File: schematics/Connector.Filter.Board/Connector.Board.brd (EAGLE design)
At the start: 160 x 100 mm, 43 parts

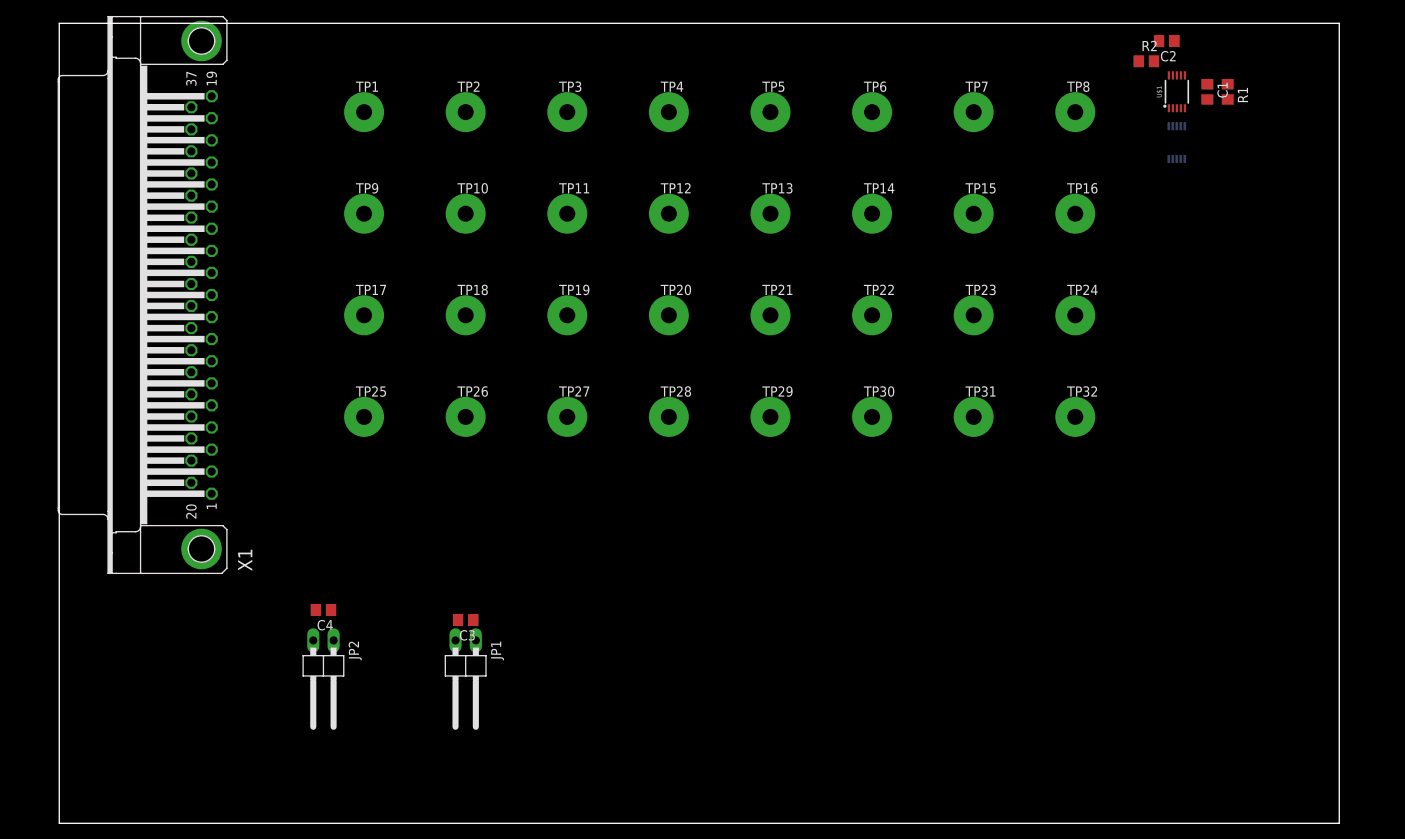
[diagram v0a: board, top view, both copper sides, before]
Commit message: example layout for 4 channels
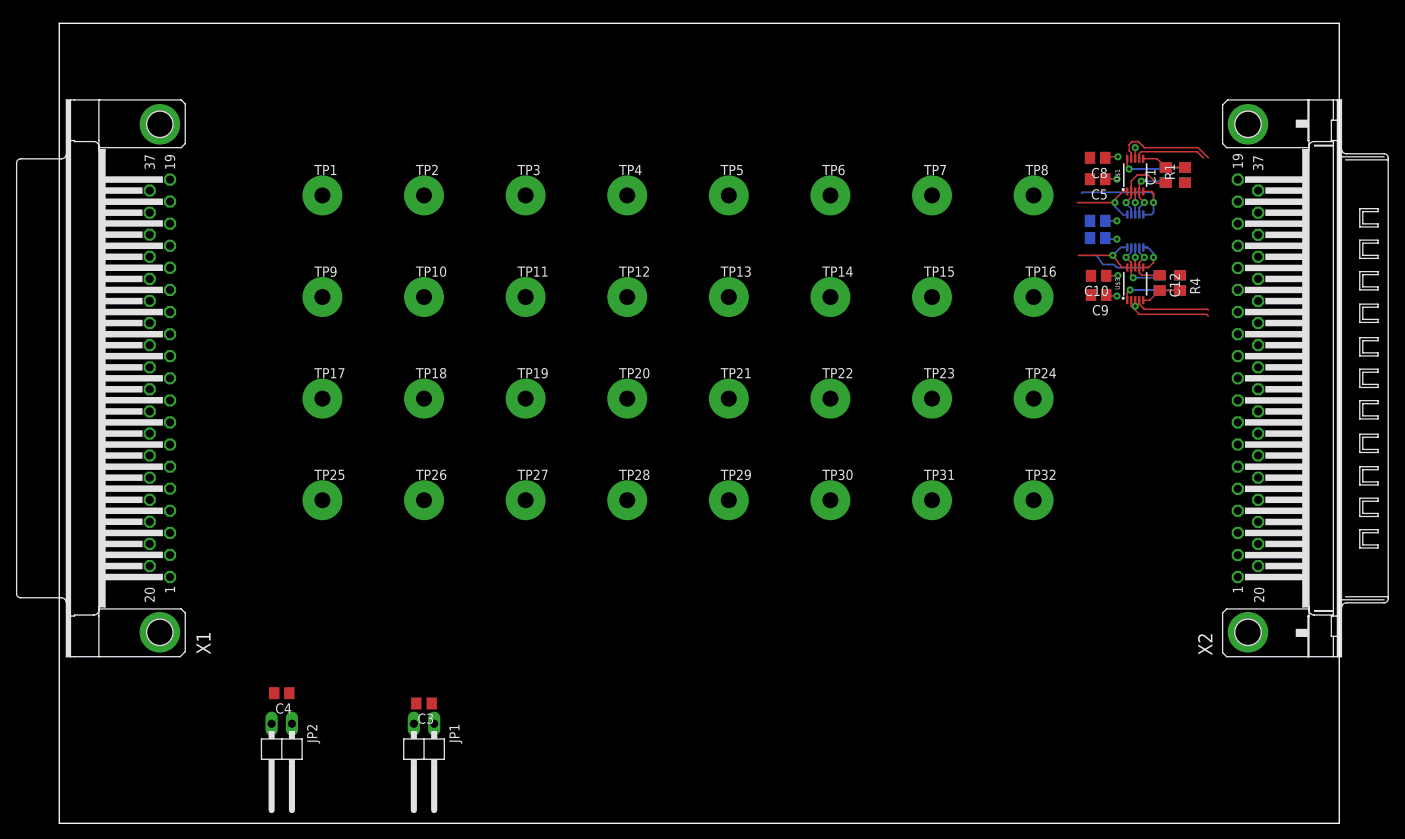
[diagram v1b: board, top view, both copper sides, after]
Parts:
- added C10, C11, C12, C5, C6, C7, C8, C9: (no value), resistor:C0805
- added R3, R4: (no value), resistor:R0805
- added U$3: AD8244, AD8244:MSOP10
- added X2: (no value), con-subd:M37HP
- moved C2 16.8 mm to (138.3, 81.0), flipped to the bottom, turned to 90 degrees
- moved R2 15.0 mm to (140.7, 81.0), flipped to the bottom, turned to 90 degrees
- moved U$2 12.2 mm to (134.5, 74.0)
- moved R1 11.7 mm to (140.7, 81.0), turned to 90 degrees
- moved X1 11.6 mm to (12.6, 55.6)
- moved C4 11.6 mm to (27.8, 16.3)
- moved JP2 11.6 mm to (27.8, 8.64)
- moved TP12 11.6 mm to (71.0, 65.8)
- moved TP13 11.6 mm to (83.7, 65.8)
- moved TP20 11.6 mm to (71.0, 53.1)
- moved TP21 11.6 mm to (83.7, 53.1)
- moved TP4 11.6 mm to (71.0, 78.5)
- moved TP5 11.6 mm to (83.7, 78.5)
- moved TP1 11.6 mm to (32.9, 78.5)
- moved TP11 11.6 mm to (58.3, 65.8)
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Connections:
- new net BUF3: C11.1, U$2.9, U$3.9
- new net BUF4: C12.1, U$2.7, U$3.7
- new net FILT10_BUF: X2.10
- new net FILT11_BUF: X2.11
- new net FILT12_BUF: X2.12
- new net FILT13_BUF: X2.13
- new net FILT14_BUF: X2.14
- new net FILT15_BUF: X2.15
- new net FILT16_BUF: X2.16
- new net FILT17_BUF: X2.17
- new net FILT18_BUF: X2.18
- new net FILT19_BUF: X2.19
- new net FILT20_BUF: X2.20
- new net FILT21_BUF: X2.21
- new net FILT22_BUF: X2.22
- new net FILT23_BUF: X2.23
- new net FILT24_BUF: X2.24
- new net FILT25_BUF: X2.25
- new net FILT26_BUF: X2.26
- new net FILT27_BUF: X2.27
- new net FILT28_BUF: X2.28
- new net FILT29_BUF: X2.29
- new net FILT30_BUF: X2.30
- new net FILT31_BUF: X2.31
- new net FILT32_BUF: X2.32
- new net FILT3_BUF: U$3.2, X2.3
- new net FILT3_OUT: C11.2, R3.2, U$3.1
- new net FILT4_BUF: U$3.4, X2.4
- new net FILT4_OUT: C12.2, R4.2, U$3.5
- new net FILT5_BUF: X2.5
- new net FILT6_BUF: X2.6
- new net FILT7_BUF: X2.7
- new net FILT8_BUF: X2.8
- new net FILT9_BUF: X2.9
- net BUF2: now also U$1.4; no longer U$1.7
- net FILT1_BUF: now also U$1.7, X2.1; no longer U$1.4
- net FILT1_OUT: now also U$1.6; no longer U$1.5
- net FILT2_BUF: now also X2.2
- net GND: now also C10.2, C5.2, C6.2, C7.2, C8.2, C9.2, R3.1, R4.1
- net PIN2: now also U$1.5; no longer U$1.6
- net PIN3: now also U$2.10, U$3.10
- net PIN4: now also U$2.6, U$3.6
- net VDD: now also C10.1, C7.1, C8.1, U$1.8, U$2.8, U$3.8; no longer U$1.3
- net VSS: now also C5.1, C6.1, C9.1, U$1.3, U$2.3, U$3.3; no longer U$1.8, U$2.8
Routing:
- net VDD: track 0.00 -> 41.2 mm, vias 0 -> 5
- net VSS: track 0.00 -> 37.6 mm, vias 0 -> 5
- net PIN2: track 0.00 -> 15.4 mm, vias 0 -> 1
- net FILT2_BUF: track 0.00 -> 12.8 mm
- net PIN4: track 0.00 -> 12.4 mm, vias 0 -> 1
- net FILT3_BUF: track 0.00 -> 10.9 mm
- net BUF1: track 0.00 -> 10.2 mm, vias 0 -> 1
- net PIN1: track 0.00 -> 9.76 mm, vias 0 -> 1
- net FILT4_BUF: track 0.00 -> 9.44 mm
- net PIN3: track 0.00 -> 9.07 mm, vias 0 -> 1
- net FILT1_BUF: track 0.00 -> 9.04 mm
- net FILT2_OUT: track 0.00 -> 8.45 mm, vias 0 -> 1
- net BUF2: track 0.00 -> 7.94 mm, vias 0 -> 2
- net BUF3: track 0.00 -> 7.86 mm, vias 0 -> 2
- net FILT3_OUT: track 0.00 -> 7.69 mm, vias 0 -> 1
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- added copper zone on layer 15, net GND

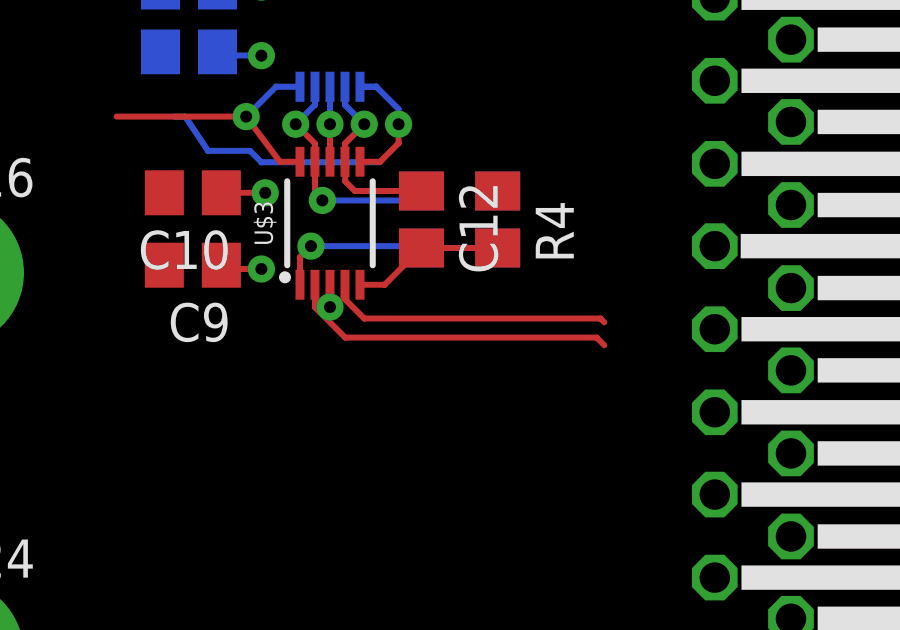
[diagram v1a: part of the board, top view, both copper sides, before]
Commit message: now passing ERC
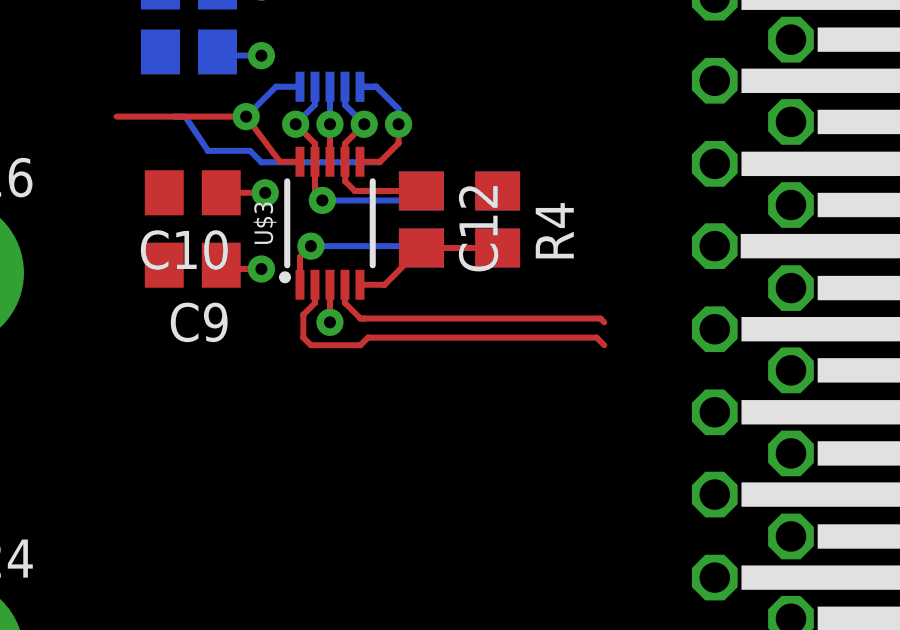
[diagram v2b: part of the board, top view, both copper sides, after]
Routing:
- net FILT3_BUF: track 10.9 -> 12.3 mm
- net VSS: track 37.6 -> 38.4 mm
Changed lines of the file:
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@@
 <contactref element="U$3" pad="3"/>
 <contactref element="C9" pad="1"/>
-<wire x1="134.493" y1="65.387" x2="134.493" y2="64.643" width="0.2" layer="1"/>
-<via x="134.493" y="64.643" extent="1-16" drill="0.4"/>
-<wire x1="134.493" y1="64.643" x2="134.493" y2="64.516" width="0.2" layer="2"/>
-<wire x1="134.493" y1="64.516" x2="132.969" y2="64.516" width="0.2" layer="2"/>
+<wire x1="134.493" y1="65.387" x2="134.493" y2="64.135" width="0.2" layer="1"/>
+<via x="134.493" y="64.135" extent="1-16" drill="0.4"/>
 <wire x1="132.969" y1="64.516" x2="132.461" y2="65.024" width="0.2" layer="2"/>
 <wire x1="132.461" y1="65.024" x2="132.461" y2="65.659" width="0.2" layer="2"/>
@@
 <wire x1="138.303" y1="74.93" x2="138.303" y2="67.056" width="0.2" layer="2"/>
 <wire x1="138.303" y1="67.056" x2="135.89" y2="64.643" width="0.2" layer="2"/>
-<wire x1="135.89" y1="64.643" x2="134.493" y2="64.643" width="0.2" layer="2"/>
 <wire x1="133.604" y1="76.708" x2="133.223" y2="76.708" width="0.2" layer="2"/>
+<wire x1="132.969" y1="64.516" x2="133.35" y2="64.135" width="0.2" layer="2"/>
+<wire x1="133.35" y1="64.135" x2="134.493" y2="64.135" width="0.2" layer="2"/>
 <wire x1="46.543" y1="14.986" x2="130.871" y2="66.04" width="0" layer="19" extent="1-1"/>
 <wire x1="46.863" y1="12.446" x2="46.543" y2="14.986" width="0" layer="19" extent="1-1"/>
+<wire x1="135.89" y1="64.643" x2="135.382" y2="64.135" width="0.2" layer="2"/>
+<wire x1="135.382" y1="64.135" x2="134.493" y2="64.135" width="0.2" layer="2"/>
 </signal>
 <signal name="FILT1_BUF">
@@
 <contactref element="X2" pad="3"/>
 <contactref element="U$3" pad="2"/>
-<wire x1="133.993" y1="65.387" x2="133.993" y2="64.635" width="0.2" layer="1"/>
-<wire x1="133.993" y1="64.635" x2="135.001" y2="63.627" width="0.2" layer="1"/>
-<wire x1="135.001" y1="63.627" x2="143.383" y2="63.627" width="0.2" layer="1"/>
 <wire x1="143.383" y1="63.627" x2="143.637" y2="63.373" width="0.2" layer="1"/>
+<wire x1="133.993" y1="65.387" x2="133.993" y2="64.778" width="0.2" layer="1"/>
+<wire x1="133.993" y1="64.778" x2="133.604" y2="64.389" width="0.2" layer="1"/>
+<wire x1="133.604" y1="64.389" x2="133.604" y2="63.627" width="0.2" layer="1"/>
+<wire x1="133.604" y1="63.627" x2="133.858" y2="63.373" width="0.2" layer="1"/>
+<wire x1="133.858" y1="63.373" x2="135.509" y2="63.373" width="0.2" layer="1"/>
 <wire x1="147.32" y1="36.2966" x2="143.637" y2="63.373" width="0" layer="19" extent="1-1"/>
+<wire x1="135.509" y1="63.373" x2="135.763" y2="63.627" width="0.2" layer="1"/>
+<wire x1="135.763" y1="63.627" x2="143.383" y2="63.627" width="0.2" layer="1"/>
 </signal>
 <signal name="FILT4_BUF">
@@
 <contactref element="U$3" pad="4"/>
 <wire x1="134.993" y1="65.387" x2="134.993" y2="64.905" width="0.2" layer="1"/>
-<wire x1="134.993" y1="64.905" x2="135.636" y2="64.262" width="0.2" layer="1"/>
 <wire x1="135.636" y1="64.262" x2="143.51" y2="64.262" width="0.2" layer="1"/>
 <wire x1="143.51" y1="64.262" x2="143.637" y2="64.135" width="0.2" layer="1"/>
+<wire x1="134.993" y1="64.905" x2="134.993" y2="64.778" width="0.2" layer="1"/>
+<wire x1="134.993" y1="64.778" x2="135.001" y2="64.77" width="0.2" layer="1"/>
+<wire x1="135.001" y1="64.77" x2="135.509" y2="64.262" width="0.2" layer="1"/>
+<wire x1="135.509" y1="64.262" x2="135.636" y2="64.262" width="0.2" layer="1"/>
 <wire x1="147.32" y1="39.0652" x2="143.637" y2="64.135" width="0" layer="19" extent="1-1"/>
 </signal>
